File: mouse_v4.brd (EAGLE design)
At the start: 100 x 65 mm, 71 parts

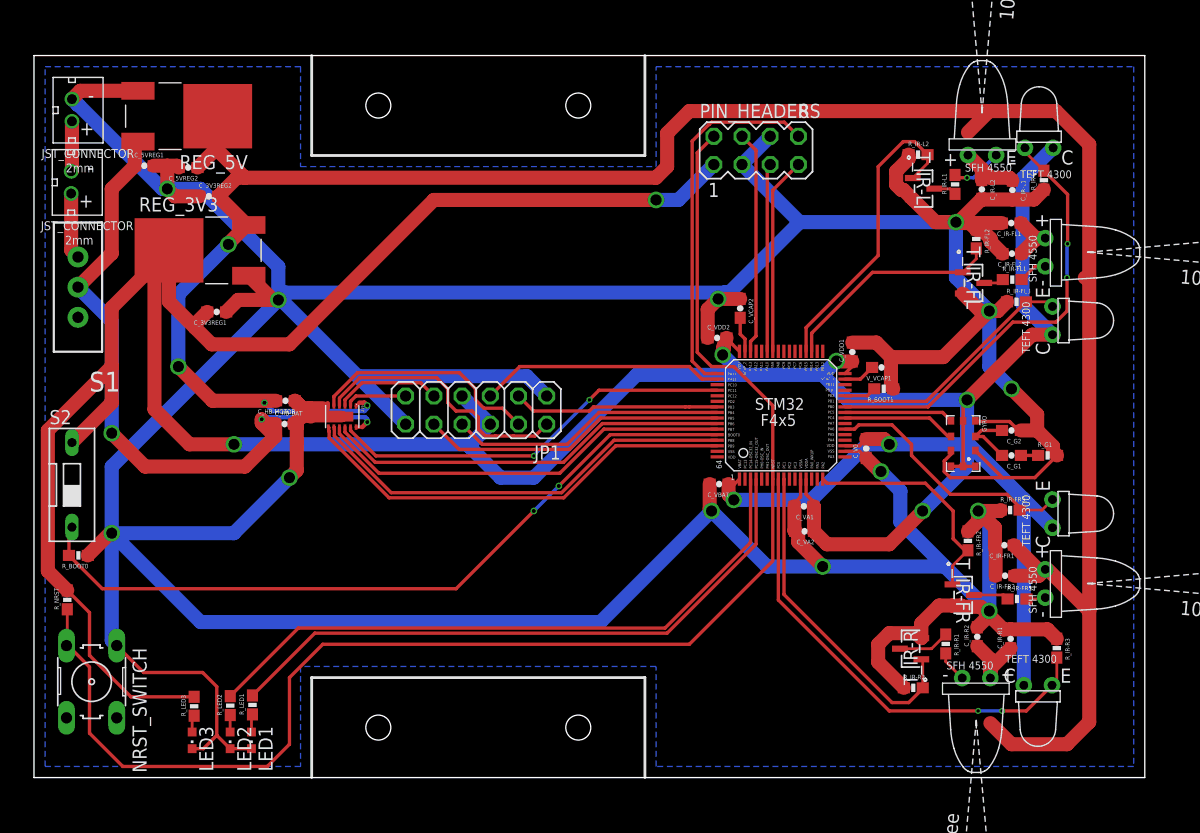
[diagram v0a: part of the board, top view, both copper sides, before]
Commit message: Added power plane
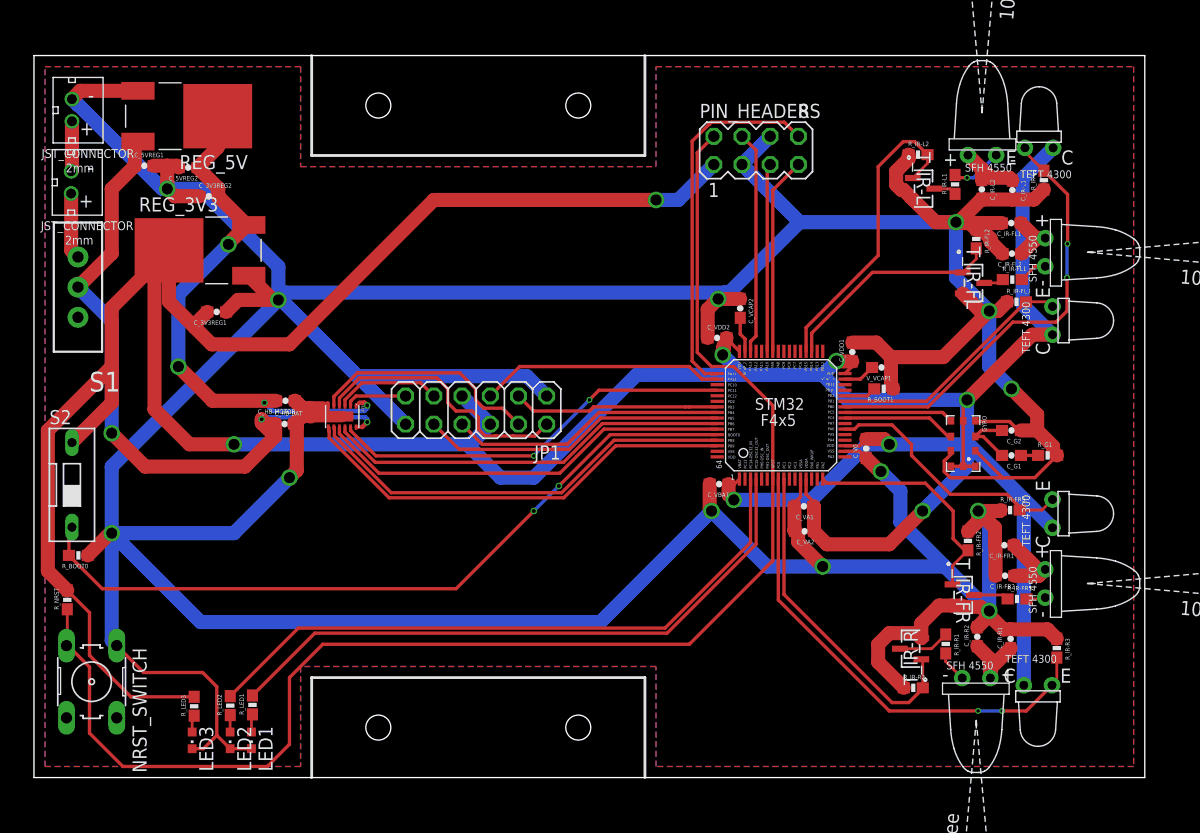
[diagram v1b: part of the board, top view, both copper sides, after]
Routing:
- net 5V: track 209.4 -> 50.7 mm
- added copper zone on layer 1, net 3V3
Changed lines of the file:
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@@
 <?xml version="1.0" encoding="utf-8"?>
 <!DOCTYPE eagle SYSTEM "eagle.dtd">
-<eagle version="9.2.2">
+<eagle version="8.6.1">
 <drawing>
 <settings>
@@
 <grid distance="1" unitdist="mm" unit="mm" style="lines" multiple="1" display="yes" altdistance="0.25" altunitdist="mm" altunit="mm"/>
 <layers>
-<layer number="1" name="Top" color="4" fill="1" visible="yes" active="yes"/>
+<layer number="1" name="Top" color="4" fill="1" visible="no" active="yes"/>
 <layer number="16" name="Bottom" color="1" fill="1" visible="yes" active="yes"/>
 <layer number="17" name="Pads" color="2" fill="1" visible="yes" active="yes"/>
@@
 <param name="checkStop" value="0"/>
 <param name="checkValues" value="0"/>
-<param name="checkNames" value="1"/>
-<param name="checkWireStubs" value="1"/>
-<param name="checkPolygonWidth" value="0"/>
 <param name="useDiameter" value="13"/>
 <param name="maxErrors" value="50"/>
@@
 <wire x1="29.75" y1="33.75" x2="30" y2="33.5" width="0.4064" layer="1"/>
 <wire x1="29.3" y1="33.75" x2="29.75" y2="33.75" width="0.4064" layer="1"/>
-<wire x1="86.1" y1="4.9" x2="88" y2="3" width="1.27" layer="1"/>
-<wire x1="93" y1="3" x2="95" y2="5" width="1.27" layer="1"/>
-<wire x1="95" y1="5" x2="95" y2="15" width="1.27" layer="1"/>
-<wire x1="95" y1="15" x2="91.26" y2="18.74" width="1.27" layer="1"/>
-<wire x1="88" y1="3" x2="93" y2="3" width="1.27" layer="1"/>
-<wire x1="95" y1="45" x2="95" y2="15" width="1.27" layer="1"/>
-<wire x1="94.6" y1="45" x2="95" y2="45" width="1.27" layer="1"/>
-<wire x1="95" y1="45" x2="95" y2="57" width="1.27" layer="1"/>
-<wire x1="95" y1="57" x2="92" y2="60" width="1.27" layer="1"/>
-<wire x1="92" y1="60" x2="86" y2="60" width="1.27" layer="1"/>
-<wire x1="86" y1="60" x2="59" y2="60" width="1.27" layer="1"/>
-<wire x1="59" y1="60" x2="57" y2="58" width="1.27" layer="1"/>
-<wire x1="57" y1="58" x2="57" y2="55" width="1.27" layer="1"/>
-<wire x1="84.08" y1="58.08" x2="86" y2="60" width="1.27" layer="1"/>
-<wire x1="57" y1="55" x2="56" y2="54" width="1.27" layer="1"/>
-<wire x1="18.26" y1="54" x2="16.59" y2="52.33" width="1.27" layer="1"/>
-<wire x1="56" y1="54" x2="19" y2="54" width="1.27" layer="1"/>
-<wire x1="19" y1="54" x2="18.26" y2="54" width="1.27" layer="1"/>
-<wire x1="16.54" y1="59.54" x2="16.54" y2="56.46" width="1.27" layer="1"/>
-<wire x1="16.54" y1="56.46" x2="19" y2="54" width="1.27" layer="1"/>
+<wire x1="14.73" y1="54.92" x2="16.59" y2="53.06" width="1.27" layer="1"/>
+<wire x1="16.59" y1="53.06" x2="16.59" y2="52.33" width="1.27" layer="1"/>
 </signal>
 <signal name="N$2">
@@
 <wire x1="86.12" y1="54" x2="85.33" y2="54.79" width="1.27" layer="1"/>
 <wire x1="87.82" y1="54" x2="86.12" y2="54" width="1.27" layer="1"/>
-<wire x1="89" y1="53.94" x2="88.08" y2="53.74" width="0" layer="19" extent="1-16"/>
-<wire x1="86.1" y1="8.96" x2="89.11" y2="8.31" width="0" layer="19" extent="1-1"/>
-<wire x1="91.04" y1="18.74" x2="91.69" y2="22.49" width="0" layer="19" extent="1-1"/>
-<wire x1="88.83" y1="49.92" x2="88.08" y2="53.74" width="0" layer="19" extent="1-1"/>
+<polygon width="0.1524" layer="1">
+<vertex x="1" y="64"/>
+<vertex x="24" y="64"/>
+<vertex x="24" y="55"/>
+<vertex x="56" y="55"/>
+<vertex x="56" y="64"/>
+<vertex x="99" y="64"/>
+<vertex x="99" y="1"/>
+<vertex x="56" y="1"/>
+<vertex x="56" y="10"/>
+<vertex x="24" y="10"/>
+<vertex x="24" y="1"/>
+<vertex x="1" y="1"/>
+</polygon>
 </signal>
 <signal name="BOOT0">
@@
 </signal>
 </signals>
-<mfgpreviewcolors>
-<mfgpreviewcolor name="soldermaskcolor" color="0xC8008000"/>
-<mfgpreviewcolor name="silkscreencolor" color="0xFFFEFEFE"/>
-<mfgpreviewcolor name="backgroundcolor" color="0xFF282828"/>
-<mfgpreviewcolor name="coppercolor" color="0xFFFFBF00"/>
-<mfgpreviewcolor name="substratecolor" color="0xFF786E46"/>
-</mfgpreviewcolors>
 </board>
 </drawing>
